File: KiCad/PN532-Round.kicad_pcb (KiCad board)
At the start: 2 copper layers, 46 x 46 mm, 52 parts, among them J1 Bell, J2 SPOX, SW1 TAMPER, U1 PN532, U2 QR, U3 QR, Y1 27.12MHz

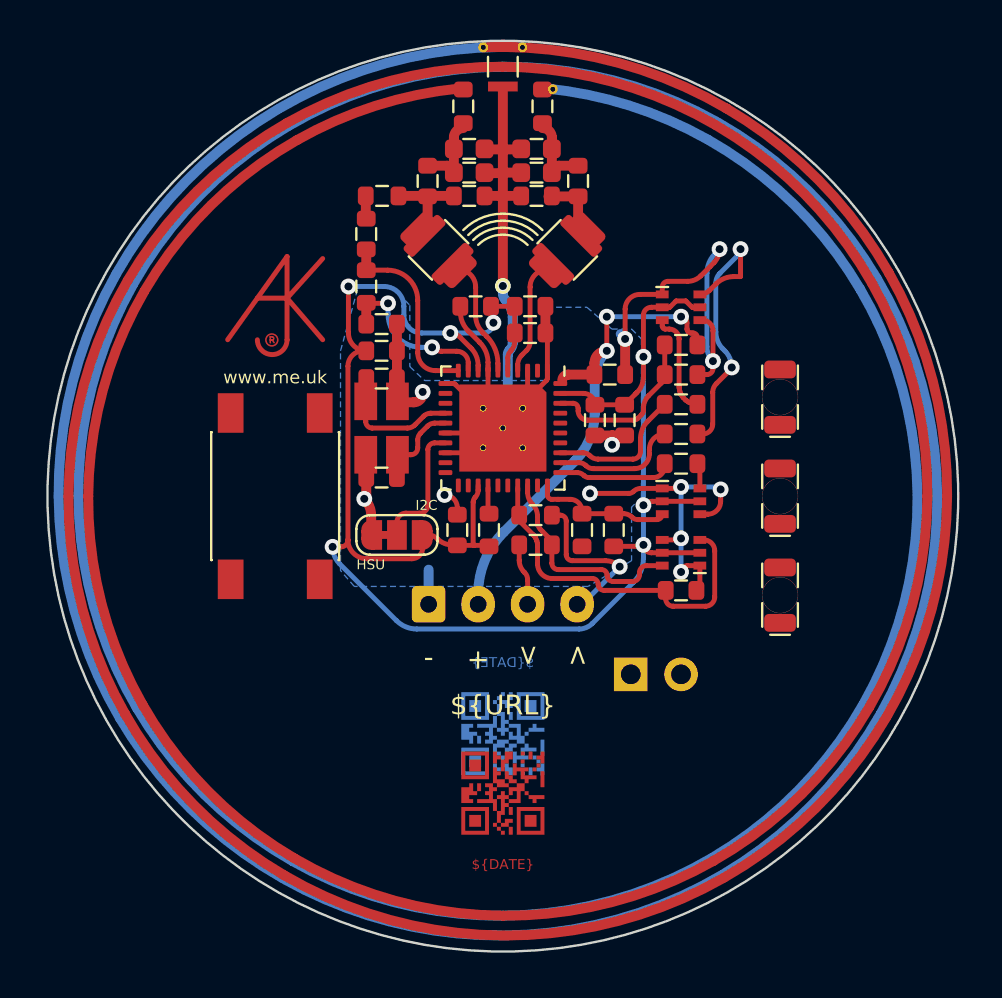
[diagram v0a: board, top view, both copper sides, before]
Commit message: New antenna design
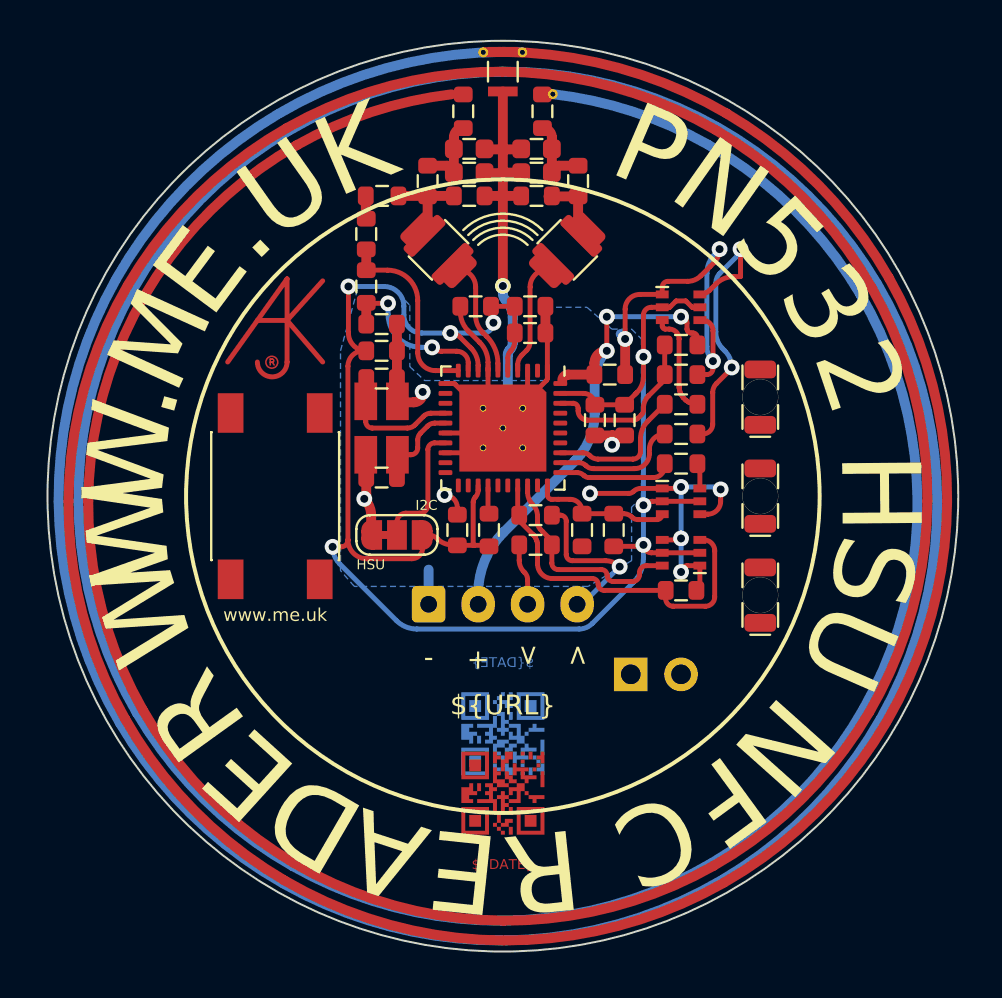
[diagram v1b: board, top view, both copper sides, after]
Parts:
- moved AJK1 1.12 mm to (89.1, 91.1)
- moved D1 1.00 mm to (113.0, 105.0)
- moved D2 1.00 mm to (113.0, 100.0)
- moved D3 1.00 mm to (113.0, 95.0)
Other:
- rule pad_to_mask_clearance: 0 -> 0.01
